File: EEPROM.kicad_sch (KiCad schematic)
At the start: 22 parts, among them IC1 PCA6408APW, IC2 AT24CS01, U2 TPS613221ADBVT

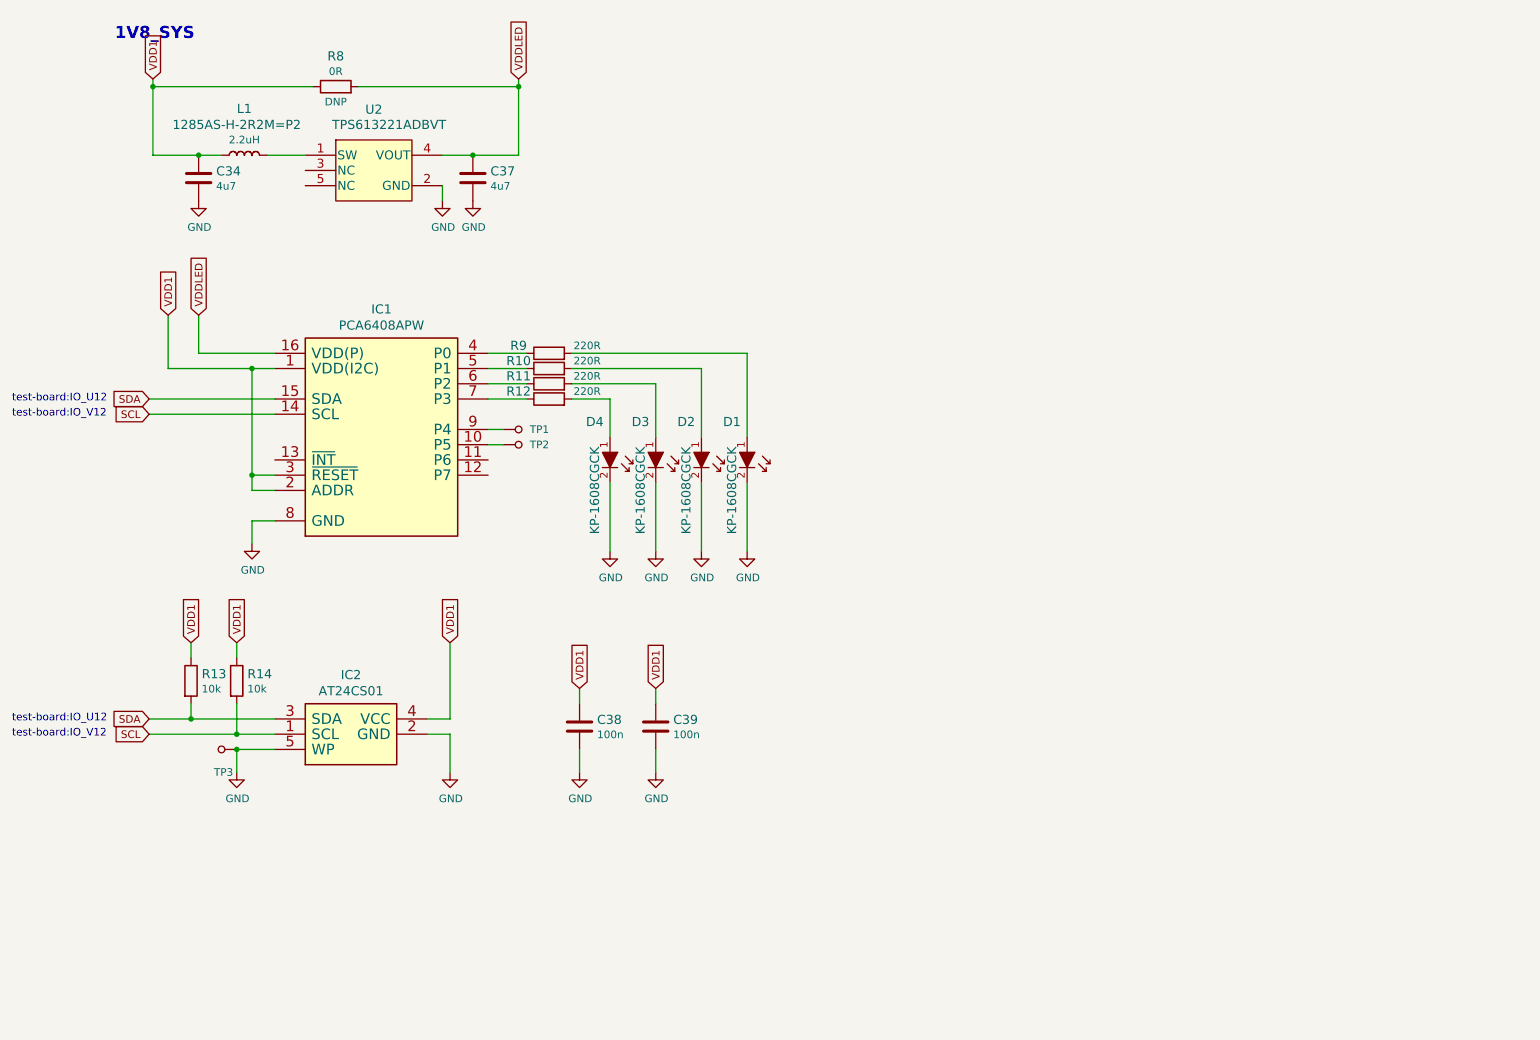
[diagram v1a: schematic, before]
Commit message: Update signage
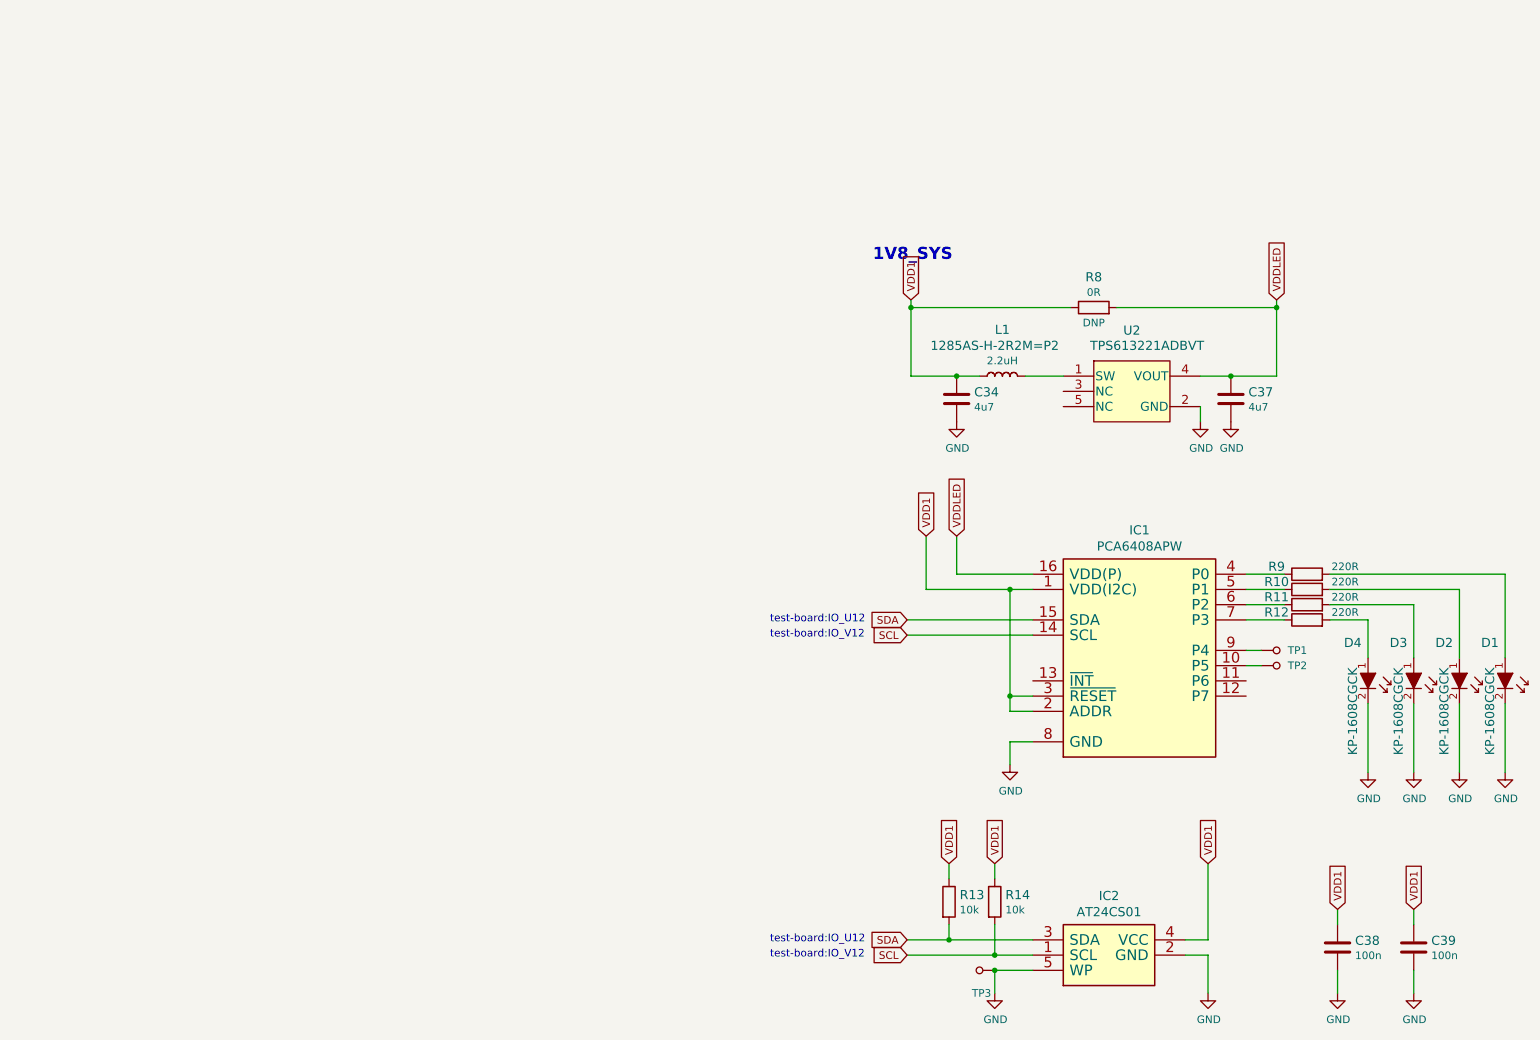
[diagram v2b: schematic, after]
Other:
- moved on the sheet: C34, C37, C38, C39, D1, D2, D3, D4, IC1, IC2, L1, R10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

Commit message: [#45231] globlib
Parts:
- C34, C37: footprint lpddr4-testbed-footprints:0402-cap -> antmicro-footprints:C_0402_1005Metric; symbol lpddr4-testbed:C_4u7_0402 -> antmicroCapacitors0402:C_4u7_0402
- C38, C39: footprint lpddr4-testbed-footprints:0402-cap -> antmicro-footprints:C_0402_1005Metric; symbol lpddr4-testbed:C_100n_0402 -> antmicroCapacitors0402:C_100n_0402
- R10, R11, R12, R9: footprint lpddr4-testbed-footprints:0402-res -> antmicro-footprints:R_0402_1005Metric; symbol lpddr4-testbed:R_220R_0402 -> antmicroResistors0402:R_220R_0402
- R13, R14: footprint lpddr4-testbed-footprints:0402-res -> antmicro-footprints:R_0402_1005Metric; symbol lpddr4-testbed:R_10k_0402 -> antmicroResistors0402:R_10k_0402
- R8: footprint lpddr4-testbed-footprints:0402-res -> antmicro-footprints:R_0402_1005Metric; symbol lpddr4-testbed:R_0R_0402 -> antmicroResistors0402:R_0R_0402
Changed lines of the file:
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@@
     )
   )
-  (symbol (lib_id "lpddr4-testbed:C_4u7_0402") (at 189.865 91.44 0) (unit 1)
+  (symbol (lib_id "antmicroCapacitors0402:C_4u7_0402") (at 189.865 91.44 0) (unit 1)
     (in_bom yes) (on_board yes)
     (property "Reference" "C34" (id 0) (at 192.786 90.297 0)
@@
       (effects (font (size 1.524 1.524)) hide)
     )
-    (property "Footprint" "lpddr4-testbed-footprints:0402-cap" (id 2) (at 194.945 86.36 0)
+    (property "Footprint" "antmicro-footprints:C_0402_1005Metric" (id 2) (at 194.945 86.36 0)
       (effects (font (size 1.524 1.524)) (justify left) hide)
     )
@@
     (pin "2")
   )
-  (symbol (lib_id "lpddr4-testbed:C_4u7_0402") (at 235.585 91.44 0) (unit 1)
+  (symbol (lib_id "antmicroCapacitors0402:C_4u7_0402") (at 235.585 91.44 0) (unit 1)
     (in_bom yes) (on_board yes)
     (property "Reference" "C37" (id 0) (at 238.506 90.297 0)
@@
       (effects (font (size 1.524 1.524)) hide)
     )
-    (property "Footprint" "lpddr4-testbed-footprints:0402-cap" (id 2) (at 240.665 86.36 0)
+    (property "Footprint" "antmicro-footprints:C_0402_1005Metric" (id 2) (at 240.665 86.36 0)
       (effects (font (size 1.524 1.524)) (justify left) hide)
     )
@@
     (pin "5")
   )
-  (symbol (lib_id "lpddr4-testbed:R_0R_0402") (at 212.725 76.2 0) (unit 1)
+  (symbol (lib_id "antmicroResistors0402:R_0R_0402") (at 212.725 76.2 0) (unit 1)
     (in_bom yes) (on_board yes)
     (property "Reference" "R8" (id 0) (at 212.725 71.12 0)
@@
       (effects (font (size 1.524 1.524)) hide)
     )
-    (property "Footprint" "lpddr4-testbed-footprints:0402-res" (id 2) (at 217.805 71.12 0)
+    (property "Footprint" "antmicro-footprints:R_0402_1005Metric" (id 2) (at 217.805 71.12 0)
       (effects (font (size 1.524 1.524)) (justify left) hide)
     )
@@
     (pin "2")
   )
-  (symbol (lib_id "lpddr4-testbed:GND") (at 189.865 95.25 0) (unit 1)
+  (symbol (lib_id "antmicropower:GND") (at 189.865 95.25 0) (unit 1)
     (in_bom yes) (on_board yes)
     (property "Reference" "#PWR0106" (id 0) (at 189.865 101.6 0)
@@
     (pin "1")
   )
-  (symbol (lib_id "lpddr4-testbed:GND") (at 235.585 95.25 0) (unit 1)
+  (symbol (lib_id "antmicropower:GND") (at 235.585 95.25 0) (unit 1)
     (in_bom yes) (on_board yes)
     (property "Reference" "#PWR0107" (id 0) (at 235.585 101.6 0)
@@
     (pin "1")
   )
-  (symbol (lib_id "lpddr4-testbed:GND") (at 230.505 95.25 0) (unit 1)
+  (symbol (lib_id "antmicropower:GND") (at 230.505 95.25 0) (unit 1)
     (in_bom yes) (on_board yes)
     (property "Reference" "#PWR0108" (id 0) (at 230.505 101.6 0)
@@
     (pin "1")
   )
-  (symbol (lib_id "lpddr4-testbed:R_10k_0402") (at 188.595 175.26 270) (unit 1)
+  (symbol (lib_id "antmicroResistors0402:R_10k_0402") (at 188.595 175.26 270) (unit 1)
     (in_bom yes) (on_board yes)
     (property "Reference" "R13" (id 0) (at 190.373 174.117 90)
@@
       (effects (font (size 1.524 1.524)) hide)
     )
-    (property "Footprint" "lpddr4-testbed-footprints:0402-res" (id 2) (at 193.675 180.34 0)
+    (property "Footprint" "antmicro-footprints:R_0402_1005Metric" (id 2) (at 193.675 180.34 0)
       (effects (font (size 1.524 1.524)) (justify left) hide)
     )
@@
     (pin "2")
   )
-  (symbol (lib_id "lpddr4-testbed:R_220R_0402") (at 248.285 120.65 0) (unit 1)
+  (symbol (lib_id "antmicroResistors0402:R_220R_0402") (at 248.285 120.65 0) (unit 1)
     (in_bom yes) (on_board yes)
     (property "Reference" "R9" (id 0) (at 243.205 119.38 0)
@@
       (effects (font (size 1.524 1.524)) hide)
     )
-    (property "Footprint" "lpddr4-testbed-footprints:0402-res" (id 2) (at 253.365 115.57 0)
+    (property "Footprint" "antmicro-footprints:R_0402_1005Metric" (id 2) (at 253.365 115.57 0)
       (effects (font (size 1.524 1.524)) (justify left) hide)
     )
@@
     (pin "2")
   )
-  (symbol (lib_id "lpddr4-testbed:R_220R_0402") (at 248.285 123.19 0) (unit 1)
+  (symbol (lib_id "antmicroResistors0402:R_220R_0402") (at 248.285 123.19 0) (unit 1)
     (in_bom yes) (on_board yes)
     (property "Reference" "R10" (id 0) (at 243.205 121.92 0)
@@
       (effects (font (size 1.524 1.524)) hide)
     )
-    (property "Footprint" "lpddr4-testbed-footprints:0402-res" (id 2) (at 253.365 118.11 0)
+    (property "Footprint" "antmicro-footprints:R_0402_1005Metric" (id 2) (at 253.365 118.11 0)
       (effects (font (size 1.524 1.524)) (justify left) hide)
     )
@@
     (pin "2")
   )
-  (symbol (lib_id "lpddr4-testbed:R_220R_0402") (at 248.285 125.73 0) (unit 1)
+  (symbol (lib_id "antmicroResistors0402:R_220R_0402") (at 248.285 125.73 0) (unit 1)
     (in_bom yes) (on_board yes)
     (property "Reference" "R11" (id 0) (at 243.205 124.46 0)
@@
       (effects (font (size 1.524 1.524)) hide)
     )
-    (property "Footprint" "lpddr4-testbed-footprints:0402-res" (id 2) (at 253.365 120.65 0)
+    (property "Footprint" "antmicro-footprints:R_0402_1005Metric" (id 2) (at 253.365 120.65 0)
       (effects (font (size 1.524 1.524)) (justify left) hide)
     )
@@
     (pin "2")
   )
-  (symbol (lib_id "lpddr4-testbed:R_220R_0402") (at 248.285 128.27 0) (unit 1)
+  (symbol (lib_id "antmicroResistors0402:R_220R_0402") (at 248.285 128.27 0) (unit 1)
     (in_bom yes) (on_board yes)
     (property "Reference" "R12" (id 0) (at 243.205 127 0)
@@
       (effects (font (size 1.524 1.524)) hide)
     )
-    (property "Footprint" "lpddr4-testbed-footprints:0402-res" (id 2) (at 253.365 123.19 0)
+    (property "Footprint" "antmicro-footprints:R_0402_1005Metric" (id 2) (at 253.365 123.19 0)
       (effects (font (size 1.524 1.524)) (justify left) hide)
     )
@@
     (pin "2")
   )
-  (symbol (lib_id "lpddr4-testbed:C_100n_0402") (at 253.365 182.88 0) (unit 1)
+  (symbol (lib_id "antmicroCapacitors0402:C_100n_0402") (at 253.365 182.88 0) (unit 1)
     (in_bom yes) (on_board yes)
     (property "Reference" "C38" (id 0) (at 256.286 181.737 0)
@@
       (effects (font (size 1.524 1.524)) hide)
     )
-    (property "Footprint" "lpddr4-testbed-footprints:0402-cap" (id 2) (at 258.445 177.8 0)
+    (property "Footprint" "antmicro-footprints:C_0402_1005Metric" (id 2) (at 258.445 177.8 0)
       (effects (font (size 1.524 1.524)) (justify left) hide)
     )
@@
     (pin "2")
   )
-  (symbol (lib_id "lpddr4-testbed:GND") (at 258.445 153.67 0) (unit 1)
+  (symbol (lib_id "antmicropower:GND") (at 258.445 153.67 0) (unit 1)
     (in_bom yes) (on_board yes)
     (property "Reference" "#PWR0109" (id 0) (at 258.445 160.02 0)
@@
     (pin "1")
   )
-  (symbol (lib_id "lpddr4-testbed:GND") (at 266.065 153.67 0) (unit 1)
+  (symbol (lib_id "antmicropower:GND") (at 266.065 153.67 0) (unit 1)
     (in_bom yes) (on_board yes)
     (property "Reference" "#PWR0110" (id 0) (at 266.065 160.02 0)
@@
     (pin "1")
   )
-  (symbol (lib_id "lpddr4-testbed:GND") (at 273.685 153.67 0) (unit 1)
+  (symbol (lib_id "antmicropower:GND") (at 273.685 153.67 0) (unit 1)
     (in_bom yes) (on_board yes)
     (property "Reference" "#PWR0111" (id 0) (at 273.685 160.02 0)
@@
     (pin "1")
   )
-  (symbol (lib_id "lpddr4-testbed:GND") (at 281.305 153.67 0) (unit 1)
+  (symbol (lib_id "antmicropower:GND") (at 281.305 153.67 0) (unit 1)
     (in_bom yes) (on_board yes)
     (property "Reference" "#PWR0112" (id 0) (at 281.305 160.02 0)
@@
     (pin "1")
   )
-  (symbol (lib_id "lpddr4-testbed:GND") (at 198.755 152.4 0) (unit 1)
+  (symbol (lib_id "antmicropower:GND") (at 198.755 152.4 0) (unit 1)
     (in_bom yes) (on_board yes)
     (property "Reference" "#PWR0113" (id 0) (at 198.755 158.75 0)
@@
     (pin "5")
   )
-  (symbol (lib_id "lpddr4-testbed:R_10k_0402") (at 196.215 175.26 270) (unit 1)
+  (symbol (lib_id "antmicroResistors0402:R_10k_0402") (at 196.215 175.26 270) (unit 1)
     (in_bom yes) (on_board yes)
     (property "Reference" "R14" (id 0) (at 197.993 174.117 90)
@@
       (effects (font (size 1.524 1.524)) hide)
     )
-    (property "Footprint" "lpddr4-testbed-footprints:0402-res" (id 2) (at 201.295 180.34 0)
+    (property "Footprint" "antmicro-footprints:R_0402_1005Metric" (id 2) (at 201.295 180.34 0)
       (effects (font (size 1.524 1.524)) (justify left) hide)
     )
@@
     (pin "2")
   )
-  (symbol (lib_id "lpddr4-testbed:GND") (at 196.215 190.5 0) (unit 1)
+  (symbol (lib_id "antmicropower:GND") (at 196.215 190.5 0) (unit 1)
     (in_bom yes) (on_board yes)
     (property "Reference" "#PWR0114" (id 0) (at 196.215 196.85 0)
@@
     (pin "1")
   )
-  (symbol (lib_id "lpddr4-testbed:GND") (at 231.775 190.5 0) (unit 1)
+  (symbol (lib_id "antmicropower:GND") (at 231.775 190.5 0) (unit 1)
     (in_bom yes) (on_board yes)
     (property "Reference" "#PWR0115" (id 0) (at 231.775 196.85 0)
@@
     (pin "1")
   )
-  (symbol (lib_id "lpddr4-testbed:GND") (at 253.365 190.5 0) (unit 1)
+  (symbol (lib_id "antmicropower:GND") (at 253.365 190.5 0) (unit 1)
     (in_bom yes) (on_board yes)
     (property "Reference" "#PWR0116" (id 0) (at 253.365 196.85 0)
@@
     (pin "1")
   )
-  (symbol (lib_id "lpddr4-testbed:C_100n_0402") (at 266.065 182.88 0) (unit 1)
+  (symbol (lib_id "antmicroCapacitors0402:C_100n_0402") (at 266.065 182.88 0) (unit 1)
     (in_bom yes) (on_board yes)
     (property "Reference" "C39" (id 0) (at 268.986 181.737 0)
@@
       (effects (font (size 1.524 1.524)) hide)
     )
-    (property "Footprint" "lpddr4-testbed-footprints:0402-cap" (id 2) (at 271.145 177.8 0)
+    (property "Footprint" "antmicro-footprints:C_0402_1005Metric" (id 2) (at 271.145 177.8 0)
       (effects (font (size 1.524 1.524)) (justify left) hide)
     )
@@
     (pin "2")
   )
-  (symbol (lib_id "lpddr4-testbed:GND") (at 266.065 190.5 0) (unit 1)
+  (symbol (lib_id "antmicropower:GND") (at 266.065 190.5 0) (unit 1)
     (in_bom yes) (on_board yes)
     (property "Reference" "#PWR0117" (id 0) (at 266.065 196.85 0)
